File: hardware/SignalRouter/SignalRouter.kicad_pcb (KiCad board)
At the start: 4 copper layers, 48 x 46 mm, 29 parts, among them J1 Src Control, J2 EXT_R, J3 EXT_L, J4 INT_R, J5 INT_L, J6 Preamp, K1 EC2-12TNU, Q1 DMN65D8L, Q10 DMN65D8L, Q2 DMN65D8L, Q3 DMN65D8L, Q4 DMP32D4S, Q5 DMN65D8L, Q6 DMN65D8L, Q7 DMP32D4S, Q8 DMN65D8L, Q9 DMN65D8L

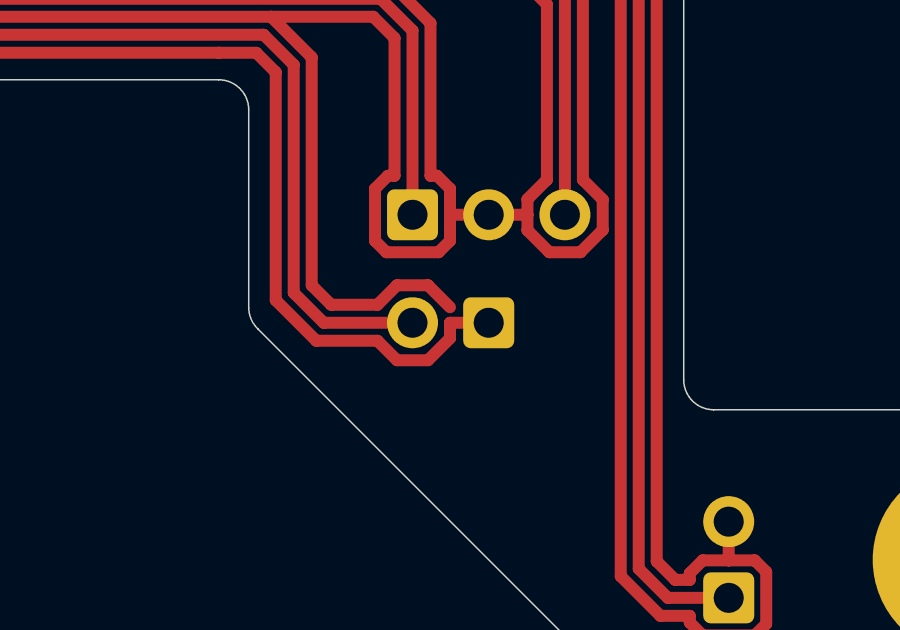
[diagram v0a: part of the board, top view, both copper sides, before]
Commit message: Completed a pile more work on the various boards that comprise the project
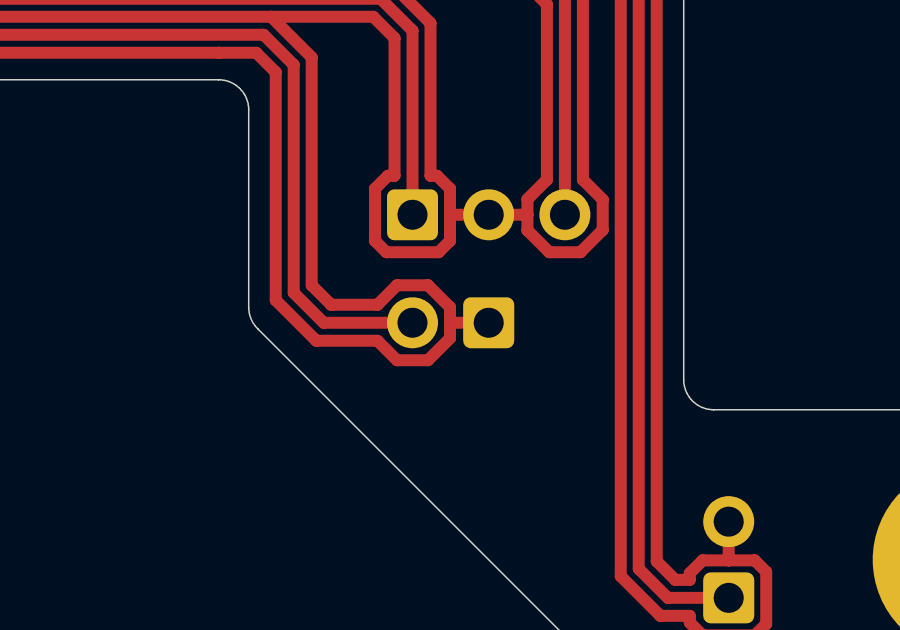
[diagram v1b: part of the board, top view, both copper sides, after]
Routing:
- net GND: track 378.3 -> 378.8 mm
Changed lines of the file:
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@@
 (kicad_pcb (version 20211014) (generator pcbnew)
   (general
-    (thickness 2.035)
+    (thickness 1.59)
   )
   (paper "A4")
@@
       (layer "F.Mask" (type "Top Solder Mask") (color "Blue") (thickness 0.01) (material "Epoxy") (epsilon_r 3.3) (loss_tangent 0))
       (layer "F.Cu" (type "copper") (thickness 0.035))
-      (layer "dielectric 1" (type "core") (thickness 0.2) (material "FR4") (epsilon_r 4.5) (loss_tangent 0.02))
+      (layer "dielectric 1" (type "core") (thickness 0.2 locked) (material "FR4") (epsilon_r 4.5) (loss_tangent 0.02))
       (layer "In1.Cu" (type "copper") (thickness 0.0175))
-      (layer "dielectric 2" (type "prepreg") (thickness 1.51) (material "FR4") (epsilon_r 4.5) (loss_tangent 0.02))
+      (layer "dielectric 2" (type "prepreg") (thickness 1.065 locked) (material "FR4") (epsilon_r 4.5) (loss_tangent 0.02))
       (layer "In2.Cu" (type "copper") (thickness 0.0175))
-      (layer "dielectric 3" (type "core") (thickness 0.2) (material "FR4") (epsilon_r 4.5) (loss_tangent 0.02))
+      (layer "dielectric 3" (type "core") (thickness 0.2 locked) (material "FR4") (epsilon_r 4.5) (loss_tangent 0.02))
       (layer "B.Cu" (type "copper") (thickness 0.035))
       (layer "B.Mask" (type "Bottom Solder Mask") (color "Blue") (thickness 0.01) (material "Epoxy") (epsilon_r 3.3) (loss_tangent 0))
@@
   (segment (start 124.641441 121.2) (end 124.21048 121.630961) (width 0.4) (layer "F.Cu") (net 17))
   (segment (start 103.40048 109.051671) (end 103.40048 115.748329) (width 0.4) (layer "F.Cu") (net 17))
+  (segment (start 126.709511 125.582435) (end 126.709511 126.1) (width 0.4) (layer "F.Cu") (net 17))
   (segment (start 105.983856 109.419511) (end 106.936144 109.419511) (width 0.4) (layer "F.Cu") (net 17))
   (segment (start 111.23 94) (end 112.520489 94) (width 0.4) (layer "F.Cu") (net 17))
